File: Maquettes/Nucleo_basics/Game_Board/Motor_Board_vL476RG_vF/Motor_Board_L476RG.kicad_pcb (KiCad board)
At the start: 2 copper layers, 120 x 110 mm, 48 parts, among them CON1 MikroE-Accelero, CON2 MikroE-nRF-S-module, J1 Speed_R, J10 Morpho_Gauche, J11 Morpho_Droite, J12 LED_1, J13 LED_2, J14 LED_3, J15 LED_4, J17 I2C_Visu, J18 I2C_EXT, J19 GND_reg, J2 Speed_L, J20 3.3V_reg, J21 MOT_R, J22 MOT_L, J23 D_IN_OUT, J3 Line_R, J4 Line_C, J5 Line_L, J6 US_Sensor, J7 Servo, J8 BAT_IN, J9 TC74A2-TempI2C, SW1 SW_1, SW2 SW_2, U1 MCP9700-Temp, U2 LM7805_TO220, U3 SN754410NE

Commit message: Update Robot Board
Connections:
- CON1 pad P3: unconnected-(CON1-CS-PadP3) -> GND
- CON1 pad P5: unconnected-(CON1-MISO-PadP5) -> GND

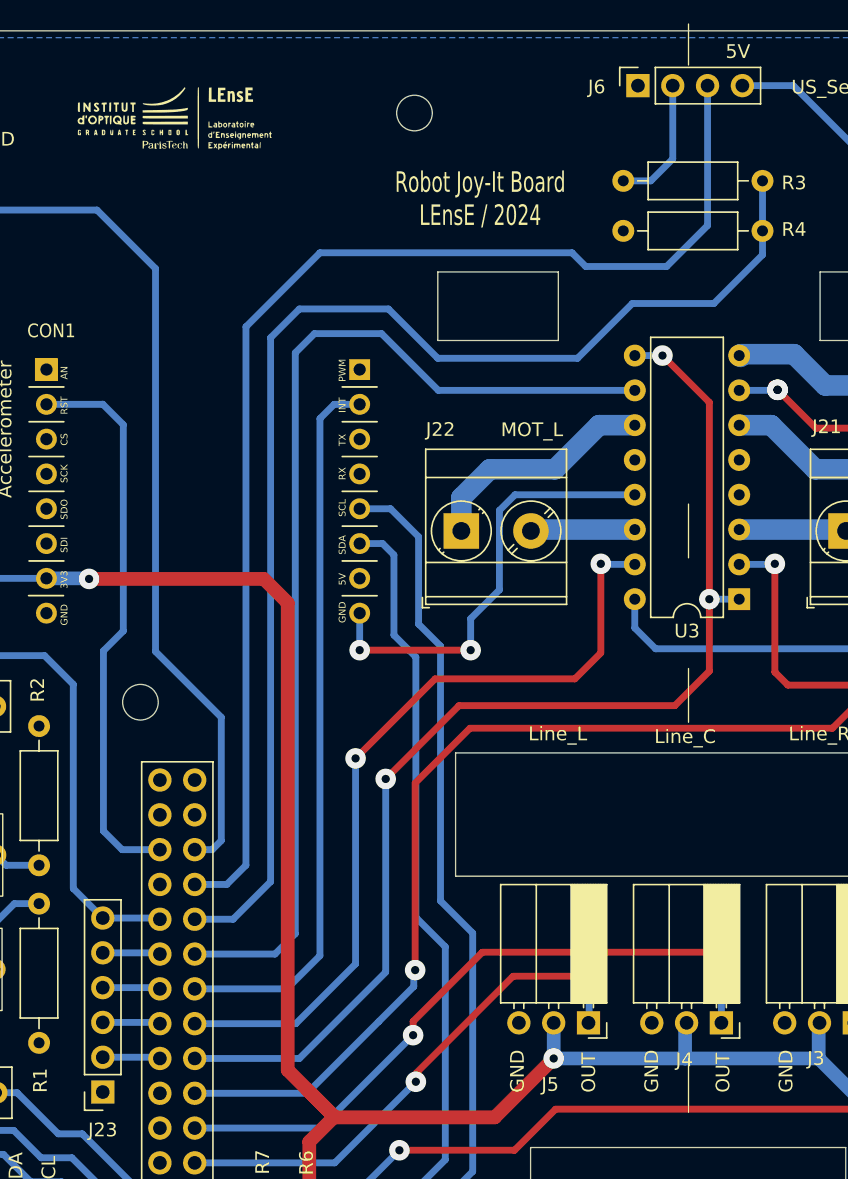
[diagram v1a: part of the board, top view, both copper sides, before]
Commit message: Update Robot Board
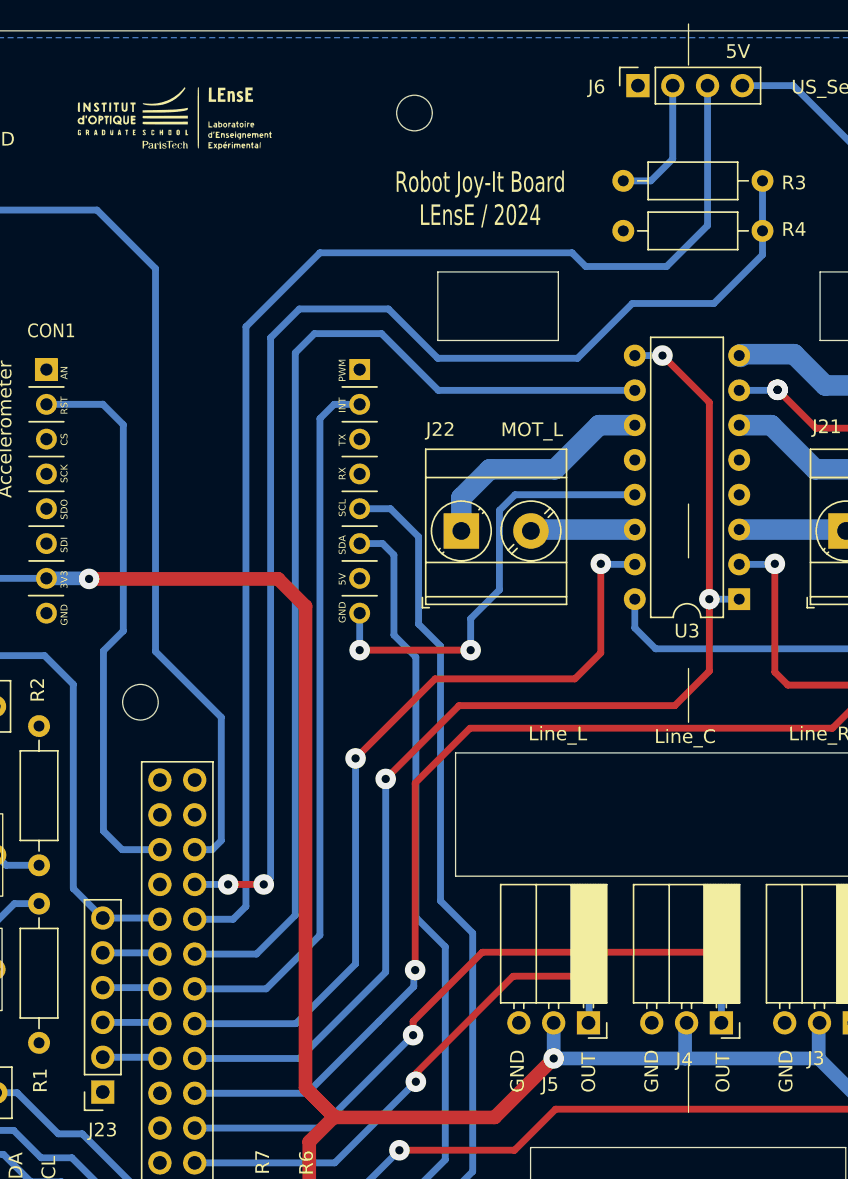
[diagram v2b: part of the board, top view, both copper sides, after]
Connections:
- J11 pad 31: US_echo_in -> US_trig
- J11 pad 33: US_trig -> US_echo_in
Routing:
- net US_trig: track 91.4 -> 94.2 mm
- net US_echo_in: track 93.2 -> 91.9 mm, vias 0 -> 2
- net Accel_INT: track 52.7 -> 51.8 mm
- net MOT_L_1: track 77.4 -> 76.6 mm
- net 3.3V_NUC: track 393.2 -> 393.8 mm
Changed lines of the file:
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@@
 			(layers "*.Cu" "*.Mask")
 			(remove_unused_layers no)
-			(net 61 "US_echo_in")
+			(net 37 "US_trig")
 			(pinfunction "Pin_31")
 			(pintype "passive")
@@
 			(layers "*.Cu" "*.Mask")
 			(remove_unused_layers no)
-			(net 37 "US_trig")
+			(net 61 "US_echo_in")
 			(pinfunction "Pin_33")
 			(pintype "passive")
@@
 	)
 	(segment
-		(start 139.75 80.5)
-		(end 152.5 80.5)
-		(width 1)
-		(layer "F.Cu")
-		(net 14)
-	)
-	(segment
-		(start 154.25 82.25)
-		(end 154.25 116.35)
+		(start 155.55 82.5)
+		(end 155.55 117.65)
 		(width 1)
 		(layer "F.Cu")
@@
 	)
 	(segment
-		(start 152.5 80.5)
-		(end 154.25 82.25)
-		(width 1)
-		(layer "F.Cu")
-		(net 14)
-	)
-	(segment
 		(start 232.5 100.75)
 		(end 232.5 114)
@@
 	)
 	(segment
-		(start 154.25 116.35)
-		(end 155.7 117.8)
+		(start 155.820001 125.7)
+		(end 152.420001 125.7)
 		(width 1)
 		(layer "F.Cu")
@@
 	)
 	(segment
-		(start 155.820001 125.7)
-		(end 152.420001 125.7)
+		(start 169.36 119.8)
+		(end 173.66 115.5)
 		(width 1)
 		(layer "F.Cu")
@@
 	)
 	(segment
-		(start 169.36 119.8)
-		(end 173.66 115.5)
+		(start 139.75 80.5)
+		(end 153.55 80.5)
 		(width 1)
 		(layer "F.Cu")
@@
 		(net 14)
 	)
+	(segment
+		(start 155.55 117.65)
+		(end 155.7 117.8)
+		(width 1)
+		(layer "F.Cu")
+		(net 14)
+	)
+	(segment
+		(start 153.55 80.5)
+		(end 155.55 82.5)
+		(width 1)
+		(layer "F.Cu")
+		(net 14)
+	)
 	(via
 		(at 139.75 80.5)
@@
 	)
 	(segment
-		(start 157.64 67.76)
-		(end 156.6 68.8)
+		(start 156.6 106.5)
+		(end 152.68 110.42)
 		(width 0.5)
 		(layer "B.Cu")
@@
 	)
 	(segment
-		(start 159.5 67.76)
-		(end 157.64 67.76)
+		(start 152.68 110.42)
+		(end 147.460001 110.42)
 		(width 0.5)
 		(layer "B.Cu")
@@
 	)
 	(segment
-		(start 154.18 110.42)
-		(end 147.460001 110.42)
+		(start 157.64 67.76)
+		(end 156.6 68.8)
 		(width 0.5)
 		(layer "B.Cu")
@@
 	)
 	(segment
-		(start 156.6 68.8)
-		(end 156.6 108)
+		(start 159.5 67.76)
+		(end 157.64 67.76)
 		(width 0.5)
 		(layer "B.Cu")
@@
 	)
 	(segment
-		(start 156.6 108)
-		(end 154.18 110.42)
+		(start 156.6 68.8)
+		(end 156.6 106.5)
 		(width 0.5)
 		(layer "B.Cu")
@@
 	)
 	(segment
-		(start 156.6 56.7)
-		(end 175 56.7)
+		(start 150.26 105.34)
+		(end 147.460001 105.34)
 		(width 0.5)
 		(layer "B.Cu")
@@
 	)
 	(segment
-		(start 181.9 57.7)
-		(end 184.89 54.71)
+		(start 156.6 56.7)
+		(end 151.2 62.1)
 		(width 0.5)
 		(layer "B.Cu")
@@
 	)
 	(segment
-		(start 149.8 102.8)
-		(end 151.2 101.4)
+		(start 151.2 62.1)
+		(end 151.2 104.4)
 		(width 0.5)
 		(layer "B.Cu")
@@
 	)
 	(segment
-		(start 151.2 62.1)
-		(end 156.6 56.7)
+		(start 176 57.7)
+		(end 175 56.7)
 		(width 0.5)
 		(layer "B.Cu")
@@
 	)
 	(segment
-		(start 151.2 101.4)
-		(end 151.2 62.1)
+		(start 175 56.7)
+		(end 156.6 56.7)
 		(width 0.5)
 		(layer "B.Cu")
@@
 	)
 	(segment
-		(start 175 56.7)
+		(start 181.9 57.7)
 		(end 176 57.7)
 		(width 0.5)
@@
 	)
 	(segment
-		(start 147.460001 102.8)
-		(end 149.8 102.8)
+		(start 184.89 54.71)
+		(end 181.9 57.7)
 		(width 0.5)
 		(layer "B.Cu")
@@
 	)
 	(segment
-		(start 184.89 54.71)
-		(end 184.89 44.5)
+		(start 151.2 104.4)
+		(end 150.26 105.34)
 		(width 0.5)
 		(layer "B.Cu")
@@
 	)
 	(segment
-		(start 176 57.7)
-		(end 181.9 57.7)
+		(start 184.89 44.5)
+		(end 184.89 54.71)
 		(width 0.5)
 		(layer "B.Cu")
@@
 	)
 	(segment
-		(start 153.32 107.88)
-		(end 154.8 106.4)
+		(start 156.2 62.6)
+		(end 161.1 62.6)
 		(width 0.5)
 		(layer "B.Cu")
@@
 	)
 	(segment
-		(start 161.1 62.6)
-		(end 165.24 66.74)
+		(start 151.97 107.88)
+		(end 154.8 105.05)
 		(width 0.5)
 		(layer "B.Cu")
@@
 	)
 	(segment
-		(start 154.8 106.4)
-		(end 154.8 64)
+		(start 165.24 66.74)
+		(end 179.58 66.74)
 		(width 0.5)
 		(layer "B.Cu")
@@
 	)
 	(segment
-		(start 165.24 66.74)
-		(end 179.58 66.74)
+		(start 154.8 105.05)
+		(end 154.8 64)
 		(width 0.5)
 		(layer "B.Cu")
@@
 	)
 	(segment
-		(start 147.460001 107.88)
-		(end 153.32 107.88)
+		(start 161.1 62.6)
+		(end 165.24 66.74)
 		(width 0.5)
 		(layer "B.Cu")
@@
 	)
 	(segment
-		(start 156.2 62.6)
-		(end 161.1 62.6)
+		(start 147.460001 107.88)
+		(end 151.97 107.88)
 		(width 0.5)
 		(layer "B.Cu")
@@
 	)
 	(segment
-		(start 185.35 60.4)
-		(end 179.4 60.4)
+		(start 149.9 102.8)
+		(end 152.5 102.8)
+		(width 0.5)
+		(layer "F.Cu")
+		(net 61)
+	)
+	(via
+		(at 149.9 102.8)
+		(size 1.5)
+		(drill 0.6)
+		(layers "F.Cu" "B.Cu")
+		(net 61)
+	)
+	(via
+		(at 152.5 102.8)
+		(size 1.5)
+		(drill 0.6)
+		(layers "F.Cu" "B.Cu")
+		(net 61)
+	)
+	(segment
+		(start 161.6 60.8)
+		(end 165.2 64.4)
 		(width 0.5)
 		(layer "B.Cu")
@@
 	)
 	(segment
-		(start 188.9 55.1)
-		(end 188.9 56.85)
+		(start 152.5 102.8)
+		(end 153 102.3)
 		(width 0.5)
 		(layer "B.Cu")
@@
 	)
 	(segment
-		(start 150.26 105.34)
-		(end 147.460001 105.34)
+		(start 188.9 56.85)
+		(end 188.9 55.1)
 		(width 0.5)
 		(layer "B.Cu")
@@
 	)
 	(segment
-		(start 161.6 60.8)
-		(end 155.1 60.8)
+		(start 175.4 64.4)
+		(end 179.4 60.4)
 		(width 0.5)
 		(layer "B.Cu")
@@
 	)
 	(segment
-		(start 155.1 60.8)
-		(end 153 62.9)
+		(start 147.460001 102.8)
+		(end 149.8 102.8)
 		(width 0.5)
 		(layer "B.Cu")
@@
 	)
 	(segment
-		(start 188.9 56.85)
-		(end 185.35 60.4)
+		(start 185.35 60.4)
+		(end 188.9 56.85)
 		(width 0.5)
 		(layer "B.Cu")
@@
 	)
 	(segment
-		(start 153 102.6)
-		(end 150.26 105.34)
+		(start 155.1 60.8)
+		(end 161.6 60.8)
 		(width 0.5)
 		(layer "B.Cu")
@@
 	)
 	(segment
-		(start 153 62.9)
-		(end 153 102.6)
+		(start 153 102.3)
+		(end 153 62.9)
 		(width 0.5)
 		(layer "B.Cu")
@@
 	)
 	(segment
-		(start 179.4 60.4)
-		(end 175.4 64.4)
+		(start 188.9 51.45)
+		(end 188.9 55.1)
 		(width 0.5)
 		(layer "B.Cu")
@@
 	)
 	(segment
-		(start 165.2 64.4)
-		(end 161.6 60.8)
+		(start 153 62.9)
+		(end 155.1 60.8)
 		(width 0.5)
 		(layer "B.Cu")
@@
 	)
 	(segment
-		(start 188.9 51.45)
-		(end 188.9 55.1)
+		(start 149.8 102.8)
+		(end 149.9 102.8)
 		(width 0.5)
 		(layer "B.Cu")
@@
 	)
 	(segment
-		(start 175.4 64.4)
-		(end 165.2 64.4)
+		(start 165.2 64.4)
+		(end 175.4 64.4)
+		(width 0.5)
+		(layer "B.Cu")
+		(net 61)
+	)
+	(segment
+		(start 179.4 60.4)
+		(end 185.35 60.4)
 		(width 0.5)
 		(layer "B.Cu")

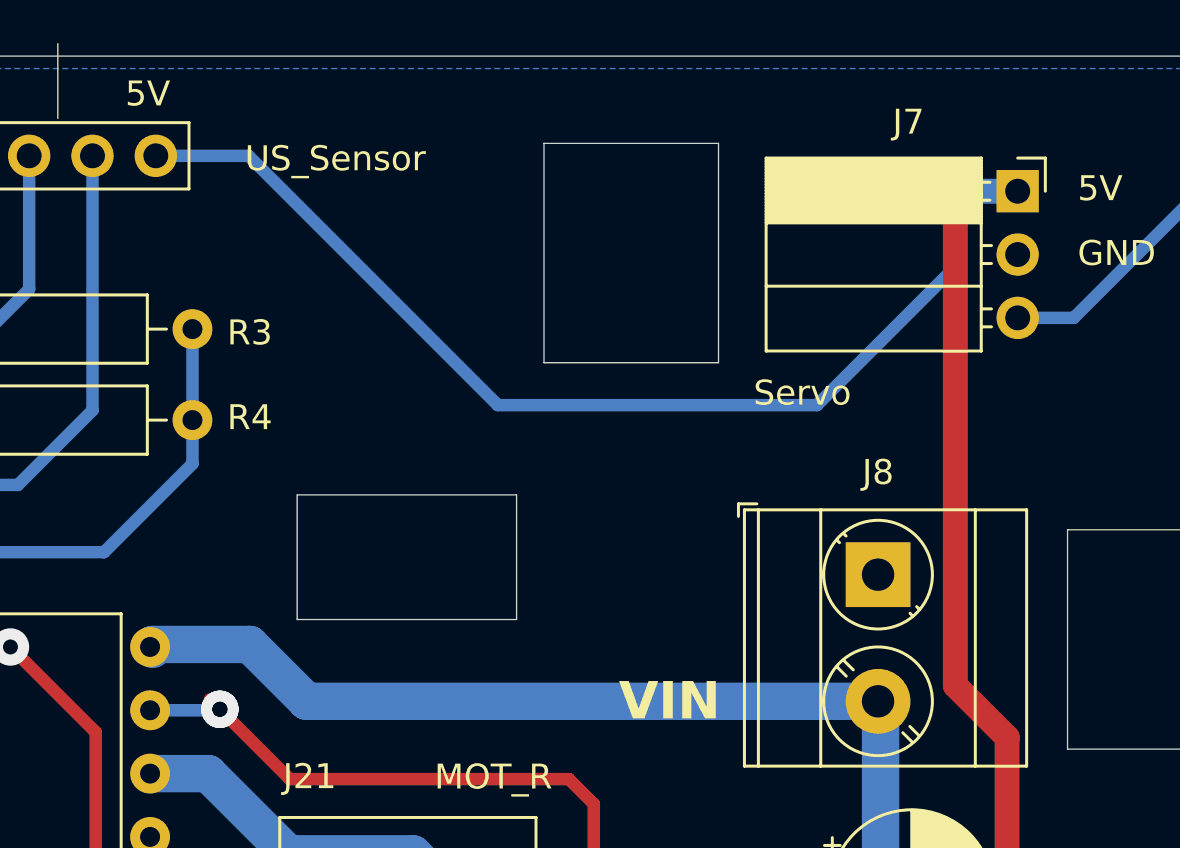
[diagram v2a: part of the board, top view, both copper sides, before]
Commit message: Update Robot and Lighting Diagram boards
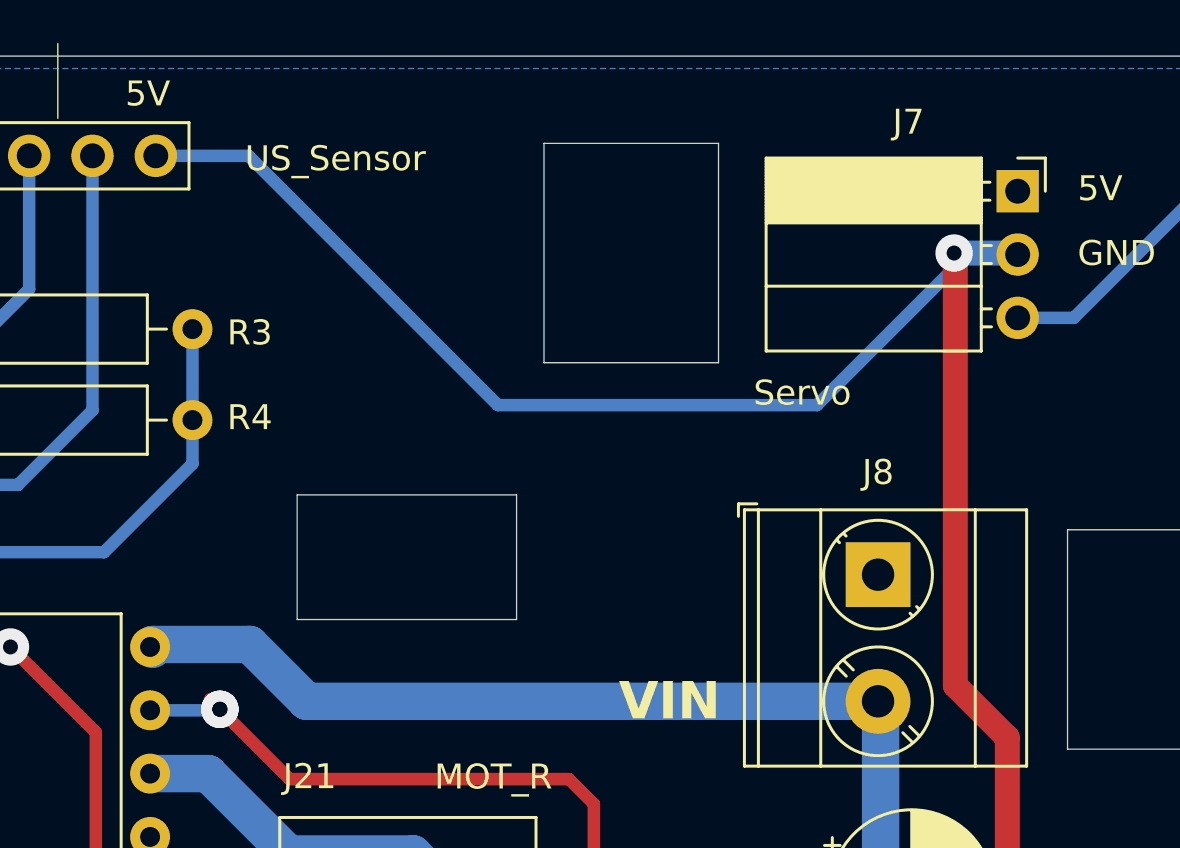
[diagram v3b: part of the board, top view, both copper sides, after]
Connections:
- J7 pad 1: 5V -> GND
- J7 pad 2: GND -> 5V
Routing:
- net 5V: track 128.8 -> 123.9 mm
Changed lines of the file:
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@@
 			(layers "*.Cu" "*.Mask")
 			(remove_unused_layers no)
-			(net 63 "5V")
+			(net 1 "GND")
 			(pinfunction "Pin_1")
 			(pintype "passive")
@@
 			(layers "*.Cu" "*.Mask")
 			(remove_unused_layers no)
-			(net 1 "GND")
+			(net 63 "5V")
 			(pinfunction "Pin_2")
 			(pintype "passive")
@@
 	)
 	(segment
-		(start 219.5 65.75)
-		(end 221.58 67.83)
+		(start 221.58 67.83)
+		(end 221.58 81)
 		(width 1)
 		(layer "F.Cu")
@@
 	)
 	(segment
-		(start 221.58 67.83)
-		(end 221.58 81)
+		(start 219.5 48.45)
+		(end 219.5 65.75)
 		(width 1)
 		(layer "F.Cu")
@@
 	)
 	(segment
-		(start 219.45 45.95)
-		(end 219.5 46)
+		(start 219.5 65.75)
+		(end 221.58 67.83)
 		(width 1)
 		(layer "F.Cu")
@@
 	)
 	(segment
-		(start 219.5 46)
-		(end 219.5 65.75)
+		(start 219.45 48.4)
+		(end 219.5 48.45)
 		(width 1)
 		(layer "F.Cu")
@@
 	)
 	(via
-		(at 219.45 45.95)
+		(at 219.45 48.4)
 		(size 1.5)
 		(drill 0.6)
@@
 	)
 	(segment
-		(start 201.15 54.5)
-		(end 213.95 54.5)
-		(width 0.5)
+		(start 179.58 81.98)
+		(end 179.36 82.2)
+		(width 1)
 		(layer "B.Cu")
 		(net 63)
 	)
 	(segment
-		(start 179.58 81.98)
-		(end 179.36 82.2)
+		(start 219.45 48.4)
+		(end 221.94 48.4)
 		(width 1)
 		(layer "B.Cu")
@@
 	)
 	(segment
-		(start 219.45 49)
-		(end 219.45 45.95)
+		(start 221.94 48.4)
+		(end 222 48.46)
+		(width 0.5)
+		(layer "B.Cu")
+		(net 63)
+	)
+	(segment
+		(start 213.95 54.5)
+		(end 201.15 54.5)
 		(width 0.5)
 		(layer "B.Cu")
@@
 	)
 	(segment
-		(start 187.43 44.5)
+		(start 201.15 54.5)
 		(end 191.15 44.5)
 		(width 0.5)
@@
 	)
 	(segment
-		(start 222 45.92)
-		(end 219.53 45.92)
-		(width 1)
-		(layer "B.Cu")
-		(net 63)
-	)
-	(segment
 		(start 191.15 44.5)
-		(end 201.15 54.5)
+		(end 187.43 44.5)
 		(width 0.5)
 		(layer "B.Cu")
@@
 	)
 	(segment
-		(start 213.95 54.5)
-		(end 219.45 49)
+		(start 219.45 49)
+		(end 213.95 54.5)
 		(width 0.5)
 		(layer "B.Cu")
@@
 	)
 	(segment
-		(start 219.5 45.95)
-		(end 219.45 45.95)
-		(width 1)
-		(layer "B.Cu")
-		(net 63)
-	)
-	(segment
-		(start 219.53 45.92)
-		(end 219.5 45.95)
-		(width 1)
+		(start 219.45 48.4)
+		(end 219.45 49)
+		(width 0.5)
 		(layer "B.Cu")
 		(net 63)
